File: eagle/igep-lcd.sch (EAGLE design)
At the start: 68 parts, among them IC1 LM1117IMPX-3.3, U1 SN74LVC8T245PW, U2 SN74LVC8T245PW, U3 SN74LVC8T245PW, U4 SN74LVC8T245PW

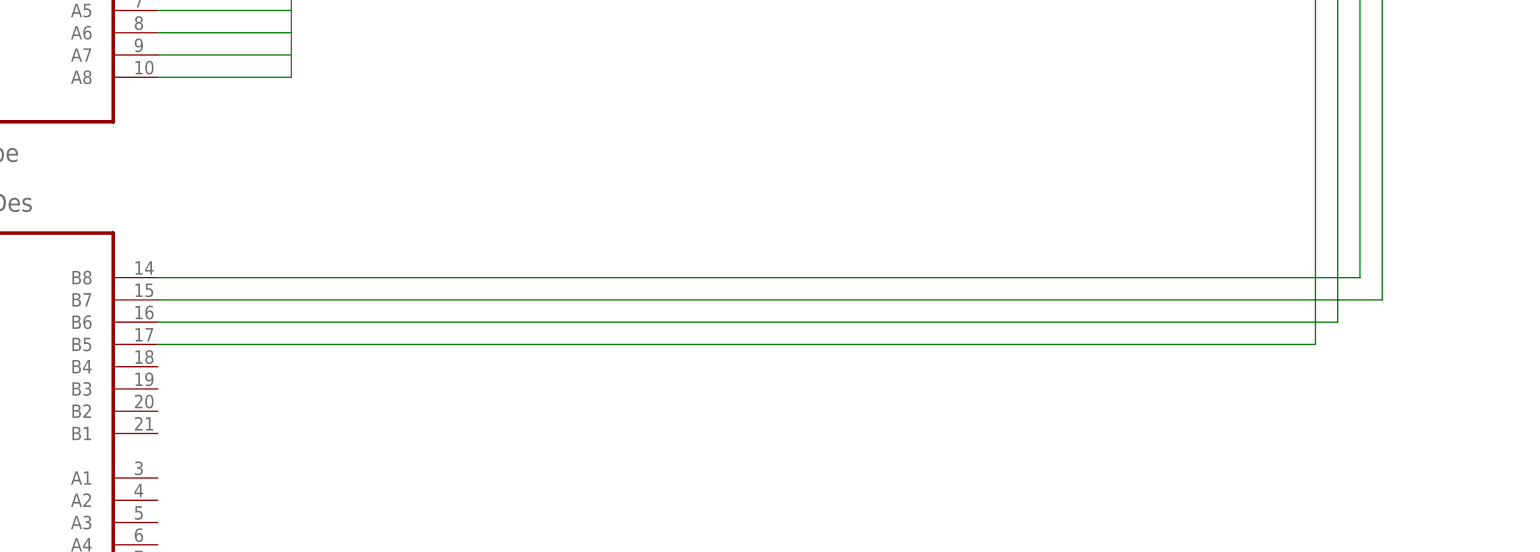
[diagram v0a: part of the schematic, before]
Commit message: Updated schematics
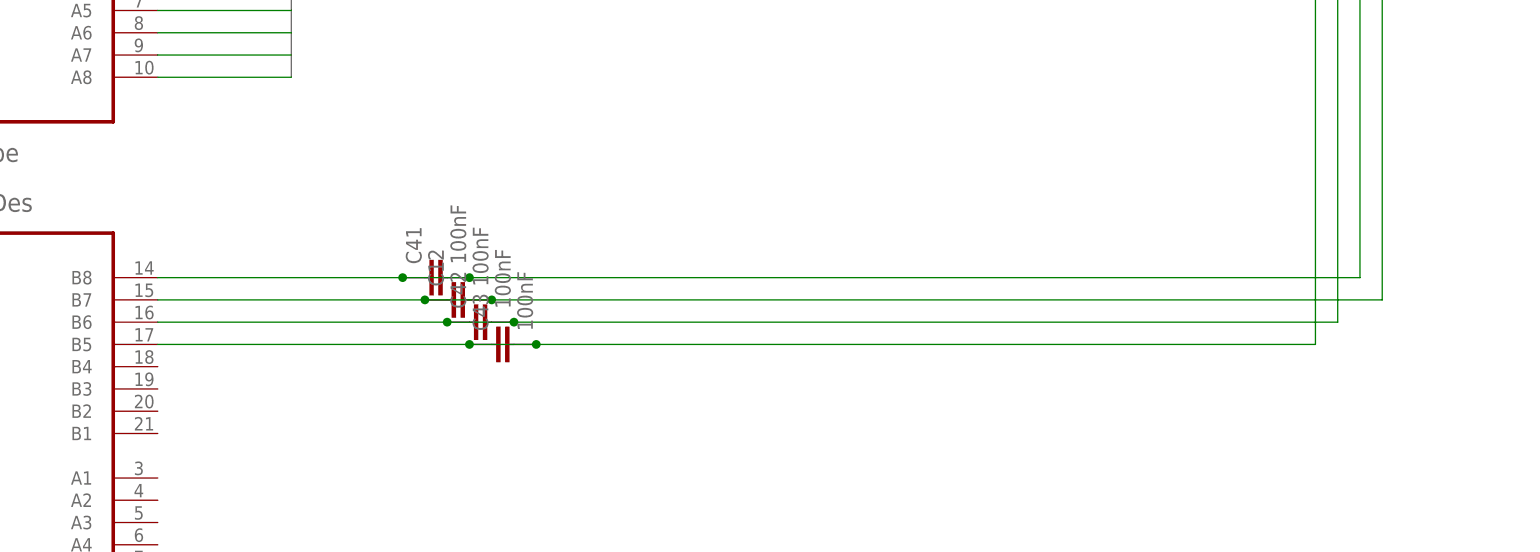
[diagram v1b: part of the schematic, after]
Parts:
- added C12, C41, C42, C43: 100nF, rcl:C-EUC1206
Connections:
- net N$10: now also C42.1, C42.2
- net N$11: now also C43.1, C43.2
- net N$5: now also C41.1, C41.2
- net N$9: now also C12.1, C12.2
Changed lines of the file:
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@@
 <part name="R9" library="rcl" deviceset="R-EU_" device="R1206" value="0"/>
 <part name="R10" library="rcl" deviceset="R-EU_" device="R1206" value="0"/>
+<part name="C12" library="rcl" deviceset="C-EU" device="C1206" value="100nF"/>
+<part name="C41" library="rcl" deviceset="C-EU" device="C1206" value="100nF"/>
+<part name="C42" library="rcl" deviceset="C-EU" device="C1206" value="100nF"/>
+<part name="C43" library="rcl" deviceset="C-EU" device="C1206" value="100nF"/>
 </parts>
 <sheets>
@@
 <instance part="R9" gate="G$1" x="78.74" y="-226.06" rot="R90"/>
 <instance part="R10" gate="G$1" x="81.28" y="-287.02" rot="R90"/>
+<instance part="C12" gate="G$1" x="208.28" y="-68.58" rot="R90"/>
+<instance part="C41" gate="G$1" x="205.74" y="-66.04" rot="R90"/>
+<instance part="C42" gate="G$1" x="210.82" y="-71.12" rot="R90"/>
+<instance part="C43" gate="G$1" x="213.36" y="-73.66" rot="R90"/>
 </instances>
 <busses>
@@
 <segment>
 <pinref part="U4" gate="A" pin="B8"/>
-<wire x1="175.26" y1="-66.04" x2="312.42" y2="-66.04" width="0.1524" layer="91"/>
+<wire x1="175.26" y1="-66.04" x2="203.2" y2="-66.04" width="0.1524" layer="91"/>
+<wire x1="203.2" y1="-66.04" x2="210.82" y2="-66.04" width="0.1524" layer="91"/>
+<wire x1="210.82" y1="-66.04" x2="312.42" y2="-66.04" width="0.1524" layer="91"/>
 <wire x1="312.42" y1="-66.04" x2="312.42" y2="10.16" width="0.1524" layer="91"/>
 <pinref part="LCD" gate="-32" pin="1"/>
 <wire x1="312.42" y1="10.16" x2="320.04" y2="10.16" width="0.1524" layer="91"/>
+<pinref part="C41" gate="G$1" pin="1"/>
+<junction x="203.2" y="-66.04"/>
+<pinref part="C41" gate="G$1" pin="2"/>
+<junction x="210.82" y="-66.04"/>
 </segment>
 </net>
@@
 <wire x1="320.04" y1="7.62" x2="314.96" y2="7.62" width="0.1524" layer="91"/>
 <pinref part="U4" gate="A" pin="B7"/>
-<wire x1="175.26" y1="-68.58" x2="314.96" y2="-68.58" width="0.1524" layer="91"/>
+<wire x1="175.26" y1="-68.58" x2="205.74" y2="-68.58" width="0.1524" layer="91"/>
+<pinref part="C12" gate="G$1" pin="1"/>
+<wire x1="205.74" y1="-68.58" x2="213.36" y2="-68.58" width="0.1524" layer="91"/>
+<junction x="205.74" y="-68.58"/>
+<pinref part="C12" gate="G$1" pin="2"/>
+<wire x1="213.36" y1="-68.58" x2="314.96" y2="-68.58" width="0.1524" layer="91"/>
+<junction x="213.36" y="-68.58"/>
 </segment>
 </net>
@@
 <segment>
 <pinref part="U4" gate="A" pin="B6"/>
-<wire x1="175.26" y1="-71.12" x2="309.88" y2="-71.12" width="0.1524" layer="91"/>
+<wire x1="175.26" y1="-71.12" x2="208.28" y2="-71.12" width="0.1524" layer="91"/>
+<wire x1="208.28" y1="-71.12" x2="215.9" y2="-71.12" width="0.1524" layer="91"/>
+<wire x1="215.9" y1="-71.12" x2="309.88" y2="-71.12" width="0.1524" layer="91"/>
 <wire x1="309.88" y1="-71.12" x2="309.88" y2="15.24" width="0.1524" layer="91"/>
 <pinref part="LCD" gate="-30" pin="1"/>
 <wire x1="309.88" y1="15.24" x2="320.04" y2="15.24" width="0.1524" layer="91"/>
+<pinref part="C42" gate="G$1" pin="1"/>
+<junction x="208.28" y="-71.12"/>
+<pinref part="C42" gate="G$1" pin="2"/>
+<junction x="215.9" y="-71.12"/>
 </segment>
 </net>
@@
 <segment>
 <pinref part="U4" gate="A" pin="B5"/>
-<wire x1="175.26" y1="-73.66" x2="307.34" y2="-73.66" width="0.1524" layer="91"/>
+<wire x1="175.26" y1="-73.66" x2="210.82" y2="-73.66" width="0.1524" layer="91"/>
+<wire x1="210.82" y1="-73.66" x2="218.44" y2="-73.66" width="0.1524" layer="91"/>
+<wire x1="218.44" y1="-73.66" x2="307.34" y2="-73.66" width="0.1524" layer="91"/>
 <wire x1="307.34" y1="-73.66" x2="307.34" y2="5.08" width="0.1524" layer="91"/>
 <pinref part="LCD" gate="-34" pin="1"/>
 <wire x1="307.34" y1="5.08" x2="320.04" y2="5.08" width="0.1524" layer="91"/>
-</segment>
-</net>
+<pinref part="C43" gate="G$1" pin="1"/>
+<junction x="210.82" y="-73.66"/>
+<pinref part="C43" gate="G$1" pin="2"/>
+<junction x="218.44" y="-73.66"/>
+</segment>
+</net>
